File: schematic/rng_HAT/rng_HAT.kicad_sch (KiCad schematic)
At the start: 33 parts, among them J1 RPi_GPIO, J2 Conn_01x04_MountingPin, Q1 2N3904, Q2 2N3904, Q3 2N3904, Q4 BC107, Q5 2N3904, U3 STM32F103C8Tx

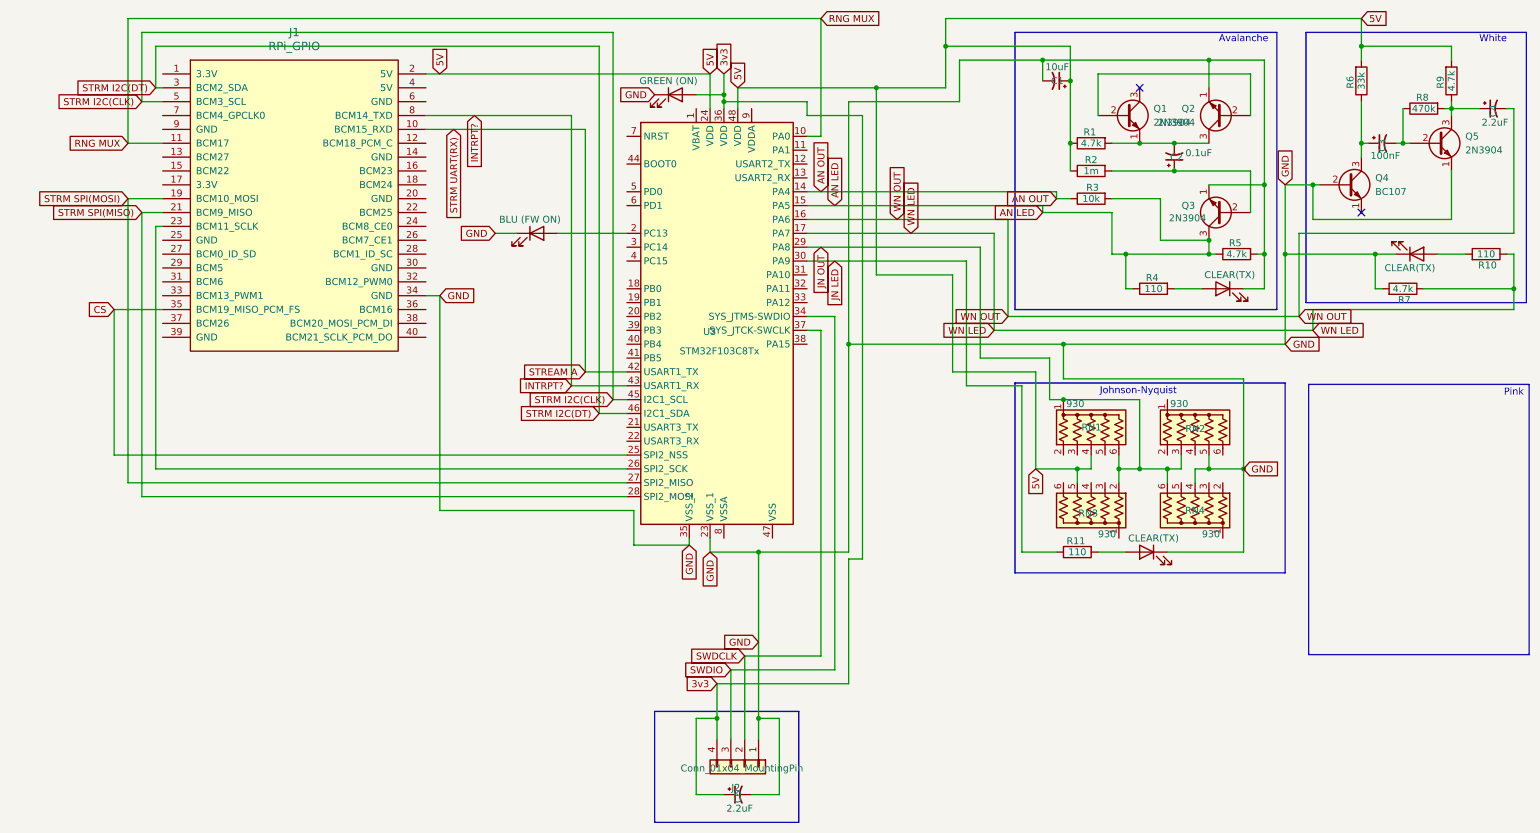
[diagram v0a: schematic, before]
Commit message: working again. small changes
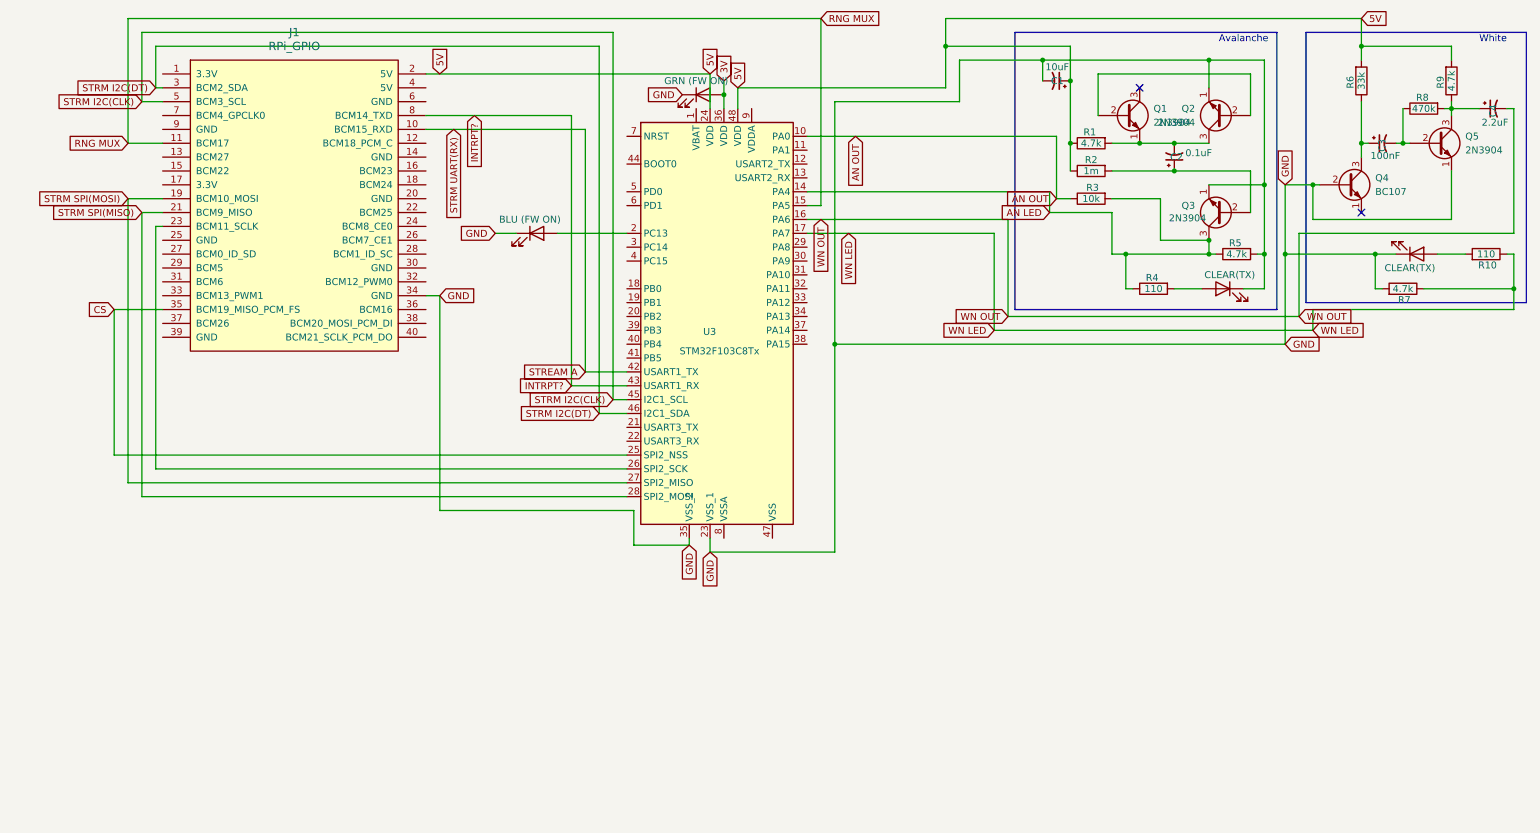
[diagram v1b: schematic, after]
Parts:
- removed C6: 2.2uF, Capacitor_SMD:CP_Elec_3x5.3, symbol Device:C_Polarized_Small_US
- removed D5: CLEAR(TX), LED_SMD:LED_0201_0603Metric, symbol Device:LED
- removed J2: Conn_01x04_MountingPin, Connector_PinHeader_1.00mm:PinHeader_1x04_P1.00mm_Horizontal, symbol Connector_Generic_MountingPin:Conn_01x04_MountingPin
- removed R11: 110, Resistor_SMD:R_0201_0603Metric, symbol Device:R
- removed RN1, RN2, RN3, RN4: 930, Resistor_THT:R_Array_SIP6, symbol Device:R_Network05_US
- D4: value GREEN (ON) -> GRN (FW ON)
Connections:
- net AN LED: now also U3.14 (PA4); no longer U3.15 (PA5)
- net AN OUT: now also U3.10 (PA0); no longer U3.14 (PA4)
- net RNG MUX: now also U3.15 (PA5); no longer U3.10 (PA0)
- net 3v3 renamed 3V
- net JN LED: no longer names the net of U3.30 (PA9)
- net JN OUT: no longer names the net of U3.29 (PA8)
- net SWDCLK: no longer names the net of U3.37 (PA14)
- net SWDIO: no longer names the net of U3.34 (PA13)
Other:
- note removed: "Johnson-Nyquist"
- note removed: "Pink"

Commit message: adding and running tests
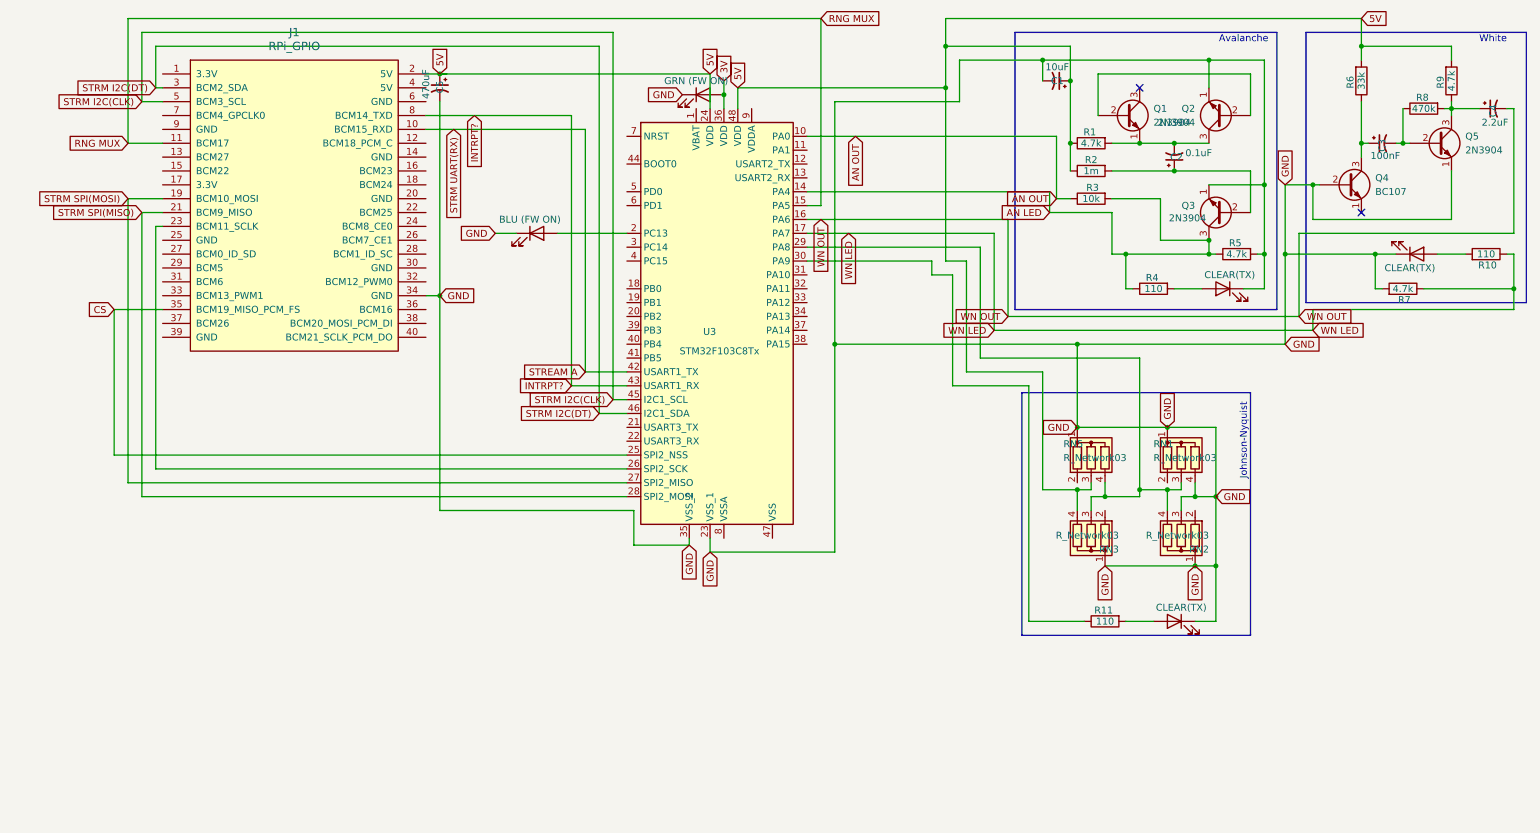
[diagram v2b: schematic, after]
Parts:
- added C5: 470uF, Capacitor_SMD:CP_Elec_3x5.3, symbol Device:C_Polarized_Small_US
- added D5: CLEAR(TX), LED_SMD:LED_0201_0603Metric, symbol Device:LED
- added R11: 110, Resistor_SMD:R_0201_0603Metric, symbol Device:R
- added RN1, RN2, RN3, RN5: R_Network03, Resistor_THT:R_Array_SIP4, symbol Device:R_Network03
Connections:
- net 5V: now also C5.1, RN3.4 (R3), RN5.3 (R2)
- net GND: now also C5.2, D5.1 (K), RN1.1 (common), RN1.4 (R3), RN2.1 (common), RN2.3 (R2), RN3.1 (common), RN5.1 (common)
- net at U3.29 (PA8): now also RN1.3 (R2), RN2.4 (R3), RN3.3 (R2), RN5.4 (R3)
- net at U3.30 (PA9): now also R11.1
- new net: D5.2 (A), R11.2
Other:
- note added: "Johnson-Nyquist"
